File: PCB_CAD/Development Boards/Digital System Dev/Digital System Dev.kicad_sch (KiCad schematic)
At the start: 65 parts, among them J1 STLINK, J10 10V, J2 PINS_LEFT, J3 3V3, J4 5V, J5 GND, J6 PINS_RIGHT, J7 DISP, J9 DC_IN, SW1 RESET, U1 STM32G474VETx, U2 DFR0570, U3 DFR0571, X1 HSE_24

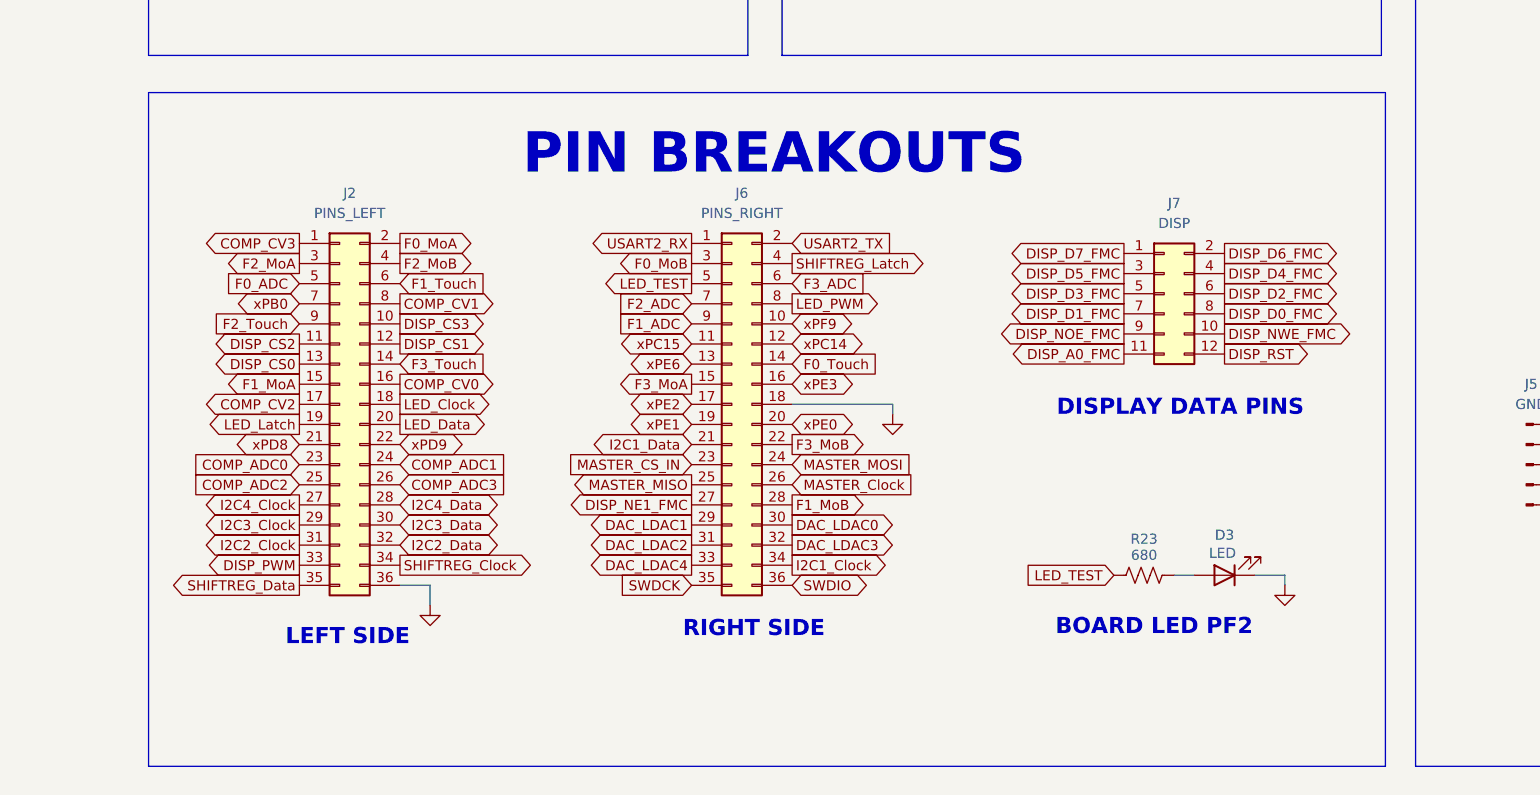
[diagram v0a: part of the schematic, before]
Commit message: extreme pcb design
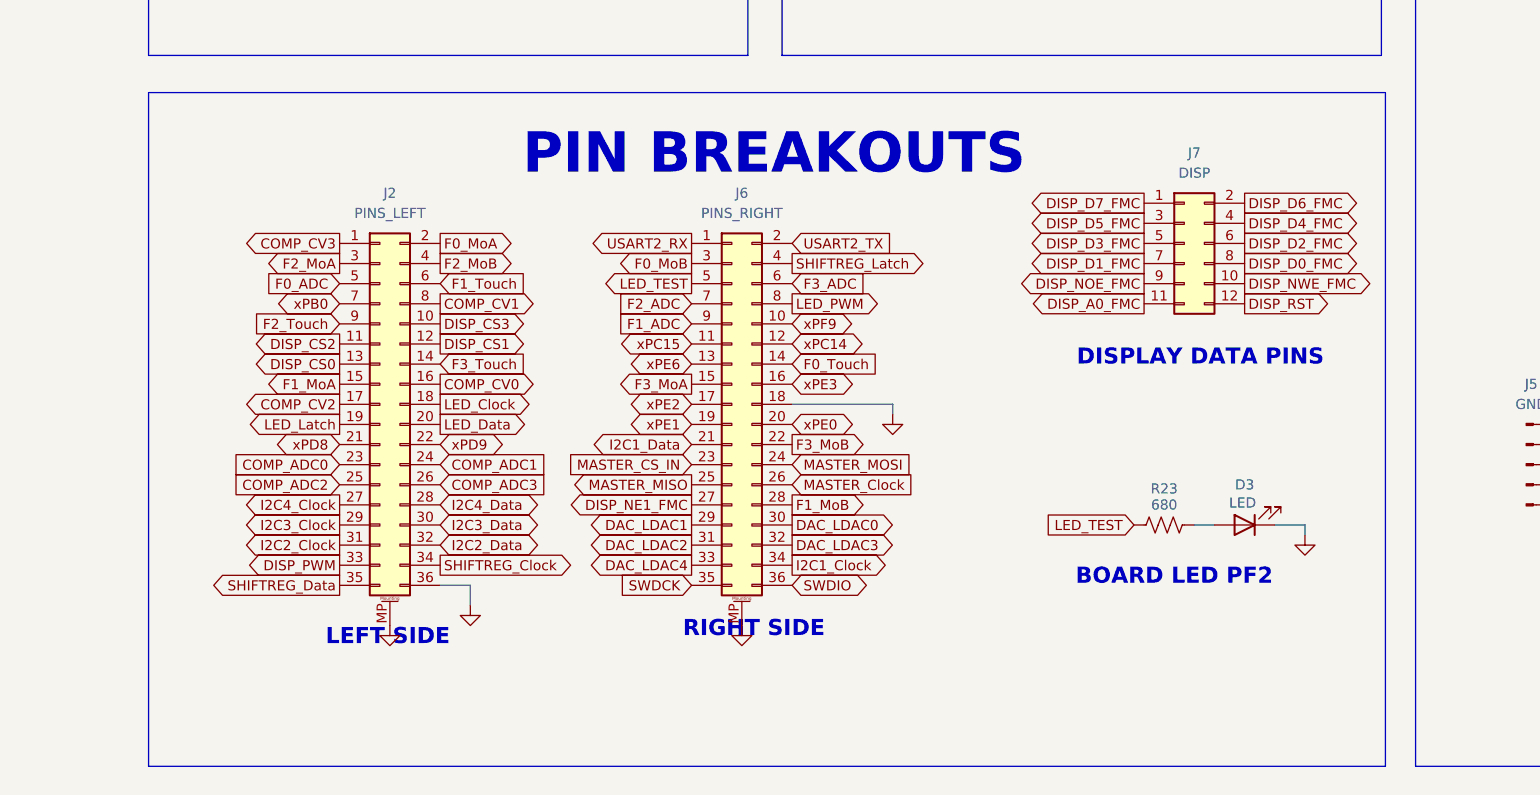
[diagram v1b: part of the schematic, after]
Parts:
- J2, J6: footprint Connector_PinHeader_2.54mm:PinHeader_2x18_P2.54mm_Vertical -> My Footprints:PinHeader_3x18_P2.54mm_Vertical_GND; symbol Connector_Generic:Conn_02x18_Odd_Even -> Connector_Generic_MountingPin:Conn_02x18_Odd_Even_MountingPin
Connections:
- net GND: now also J2.MP (MountPin), J6.MP (MountPin)
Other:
- moved on the sheet: D3, J7, R23
